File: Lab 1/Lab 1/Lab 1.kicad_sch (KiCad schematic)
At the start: 24 parts, among them K1 Fujitsu_FTR-LYCA005x, K2 Fujitsu_FTR-LYCA005x, K3 Fujitsu_FTR-LYCA005x, K4 Fujitsu_FTR-LYCA005x, K5 Fujitsu_FTR-LYCA005x, K6 Fujitsu_FTR-LYCA005x, K7 Fujitsu_FTR-LYCA005x, M1 Motor_DC, SW1 SW_Push, SW2 SW_Push_Open, SW3 SW_Push, SW4 SW_Push_Open, SW5 SW_Push, SW6 SW_Push

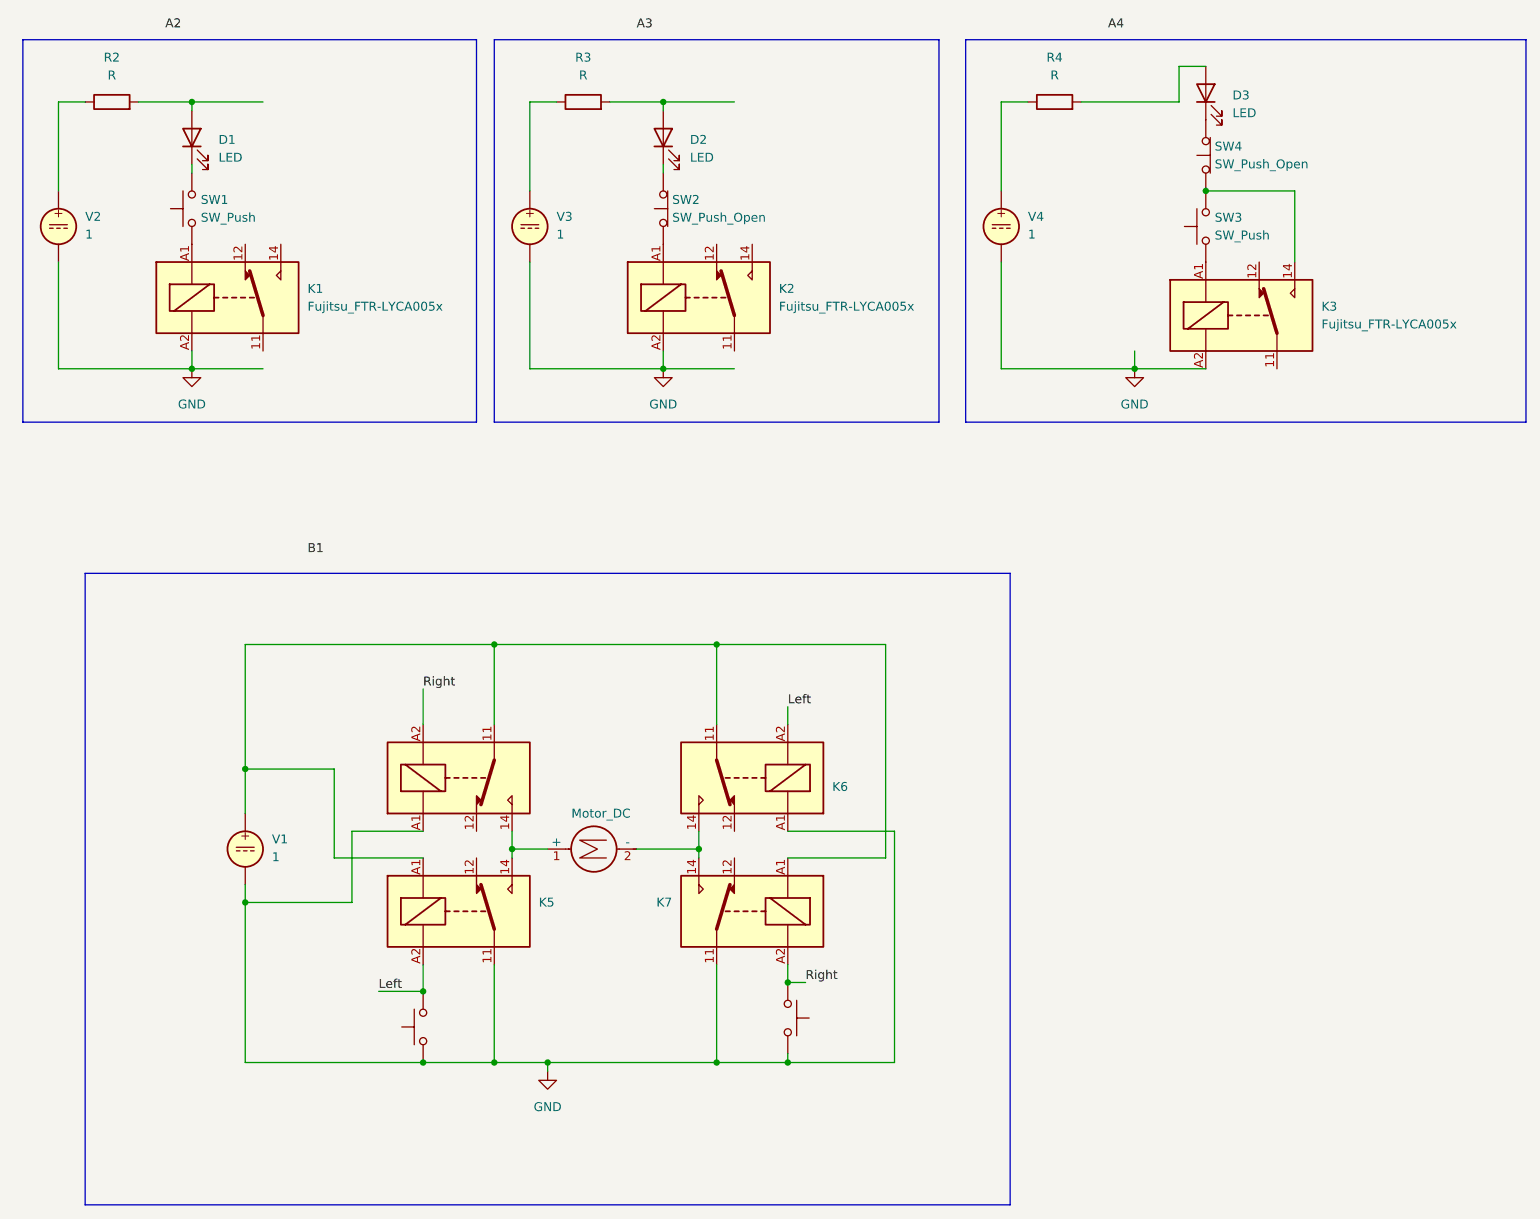
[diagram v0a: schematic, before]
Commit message: Fix B1
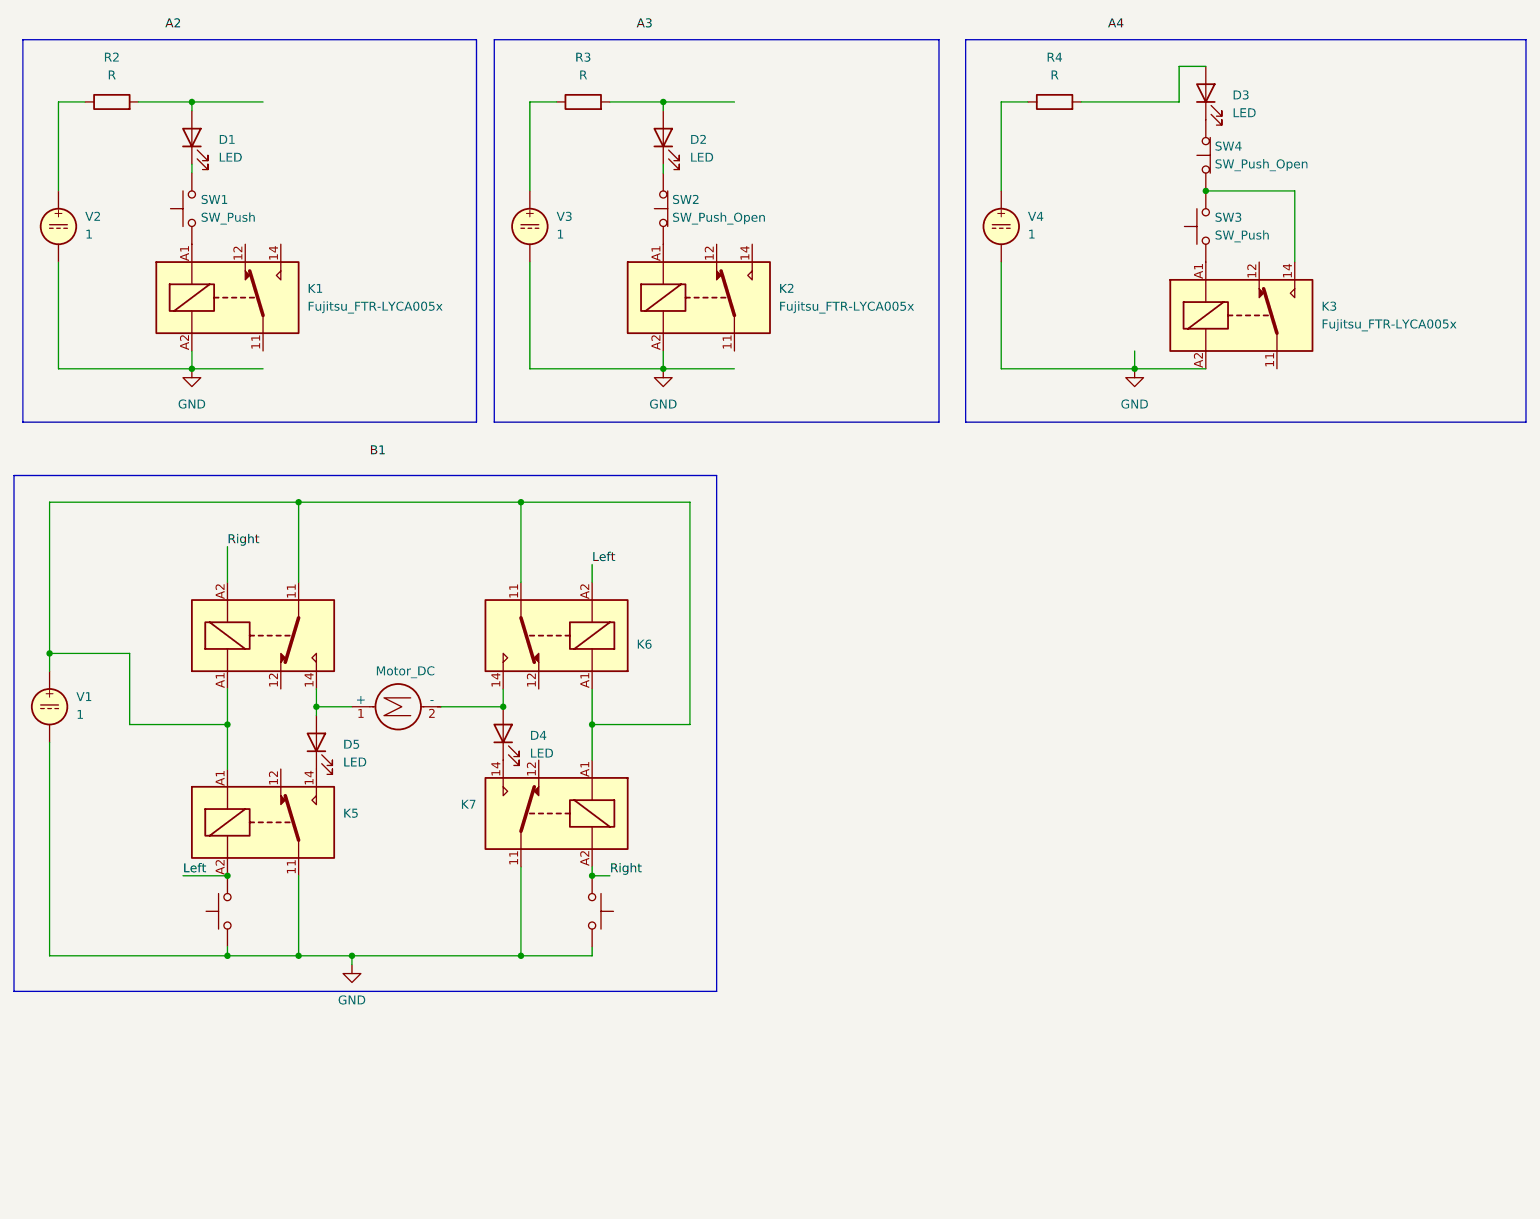
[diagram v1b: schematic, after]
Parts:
- added D4, D5: LED, symbol Device:LED
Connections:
- net GND: no longer K4.A1, K6.A1
- net at K4.11, K5.A1, K6.11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: now also K4.A1, K6.A1
- net at K6.14, M1.2 (-): now also D4.2 (A); no longer K7.14
- net at K4.14, M1.1 (+): now also D5.2 (A); no longer K5.14
- new net: D5.1 (K), K5.14
- new net: D4.1 (K), K7.14
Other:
- moved on the sheet: K5, K6, K7, V1
